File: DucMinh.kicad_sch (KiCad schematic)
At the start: 62 parts, among them J1 Power, J10 HC05, J11 PWR_Selection, J12 BOOT0, J2 M1, J3 USB_B_Micro, J4 M2, J5 M3, J6 AS5600, J7 STLink, J8 Stepper_Motor, SW1 SW_Push, U10 BTS7960B, U2 AMS1117-3.3, U3 LM2596SX-5.0/NOPB, U4 TMC2209_SILENTSTEPSTICK, U5 BTS7960B, U6 STM32F103RCT6, U8 BTS7960B, Y1 8 MHz

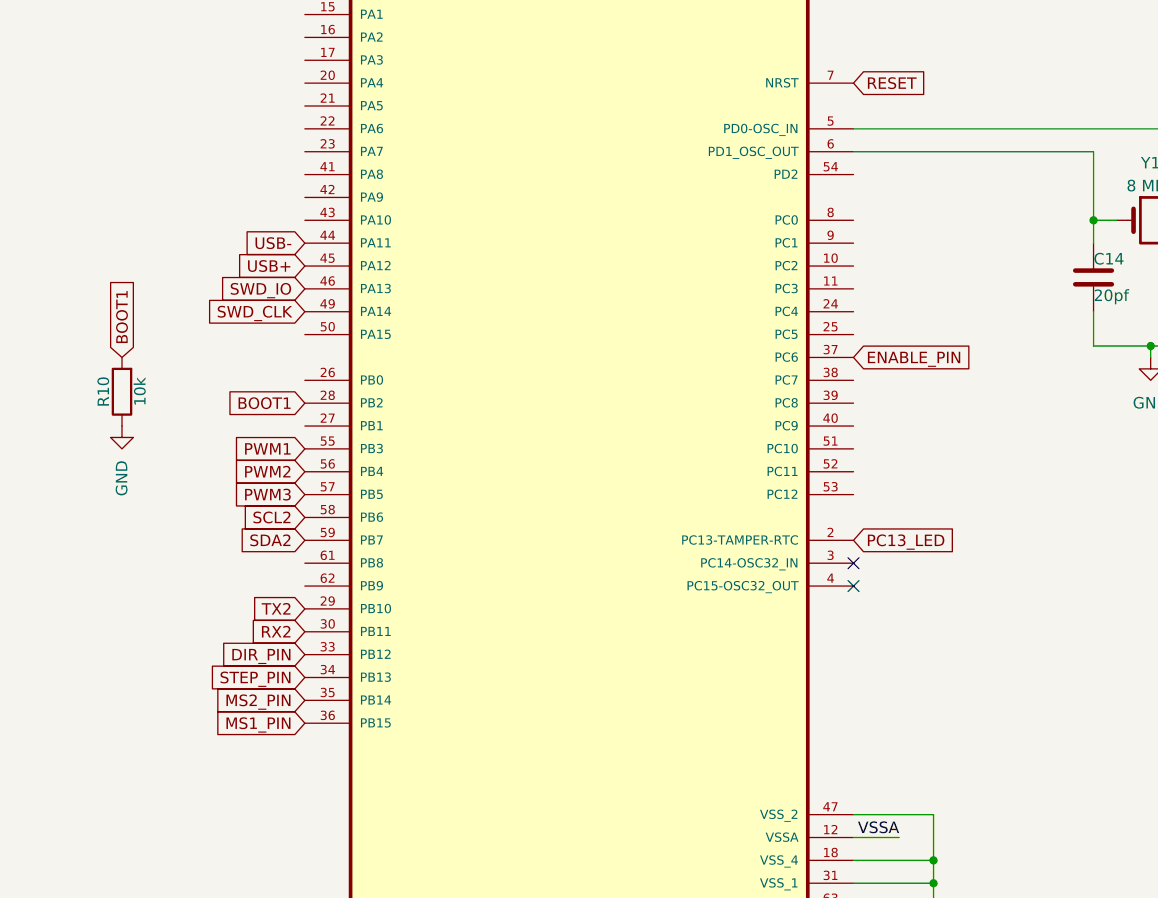
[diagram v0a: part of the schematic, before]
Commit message: final2
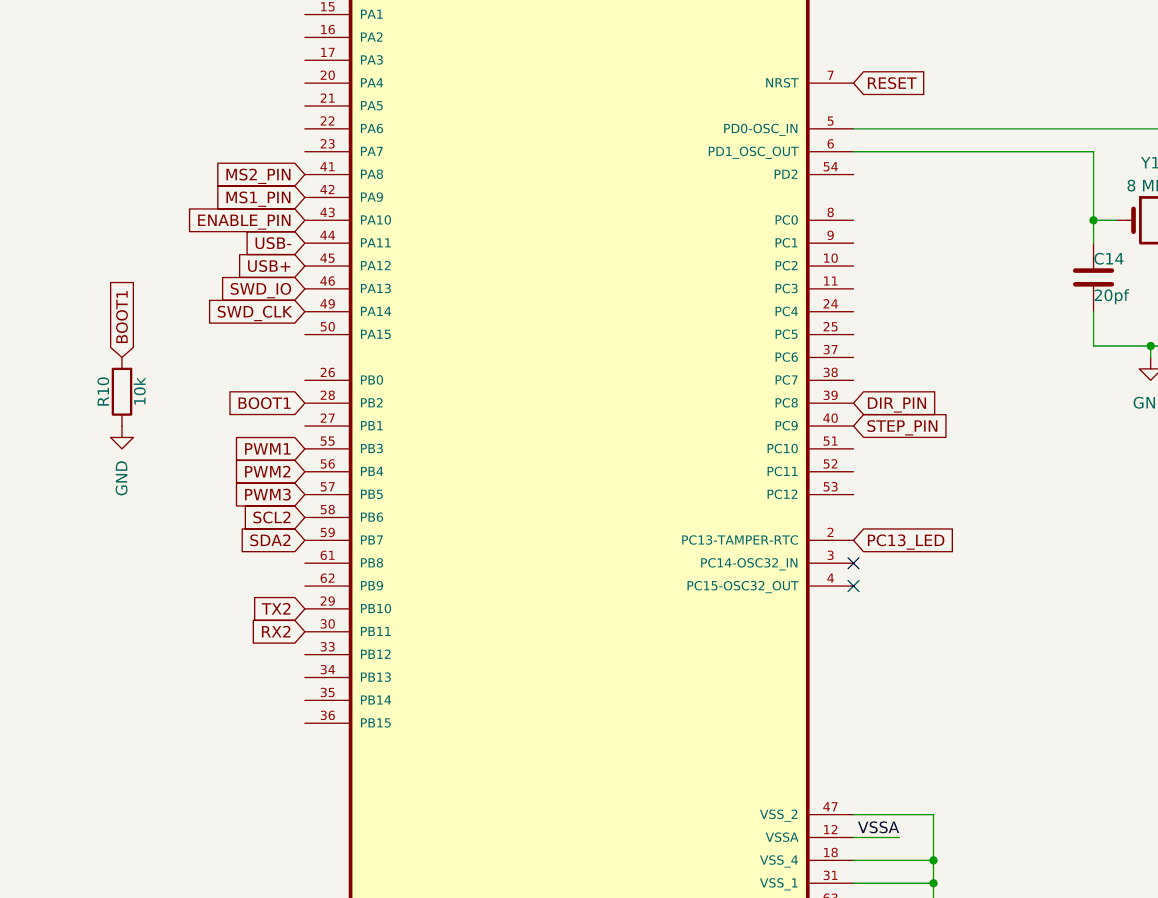
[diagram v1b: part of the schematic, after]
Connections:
- net DIR_PIN: now also U6.39 (PC8); no longer U6.33 (PB12)
- net ENABLE_PIN: now also U6.43 (PA10); no longer U6.37 (PC6)
- net MS1_PIN: now also U6.42 (PA9); no longer U6.36 (PB15)
- net MS2_PIN: now also U6.41 (PA8); no longer U6.35 (PB14)
- net STEP_PIN: now also U6.40 (PC9); no longer U6.34 (PB13)
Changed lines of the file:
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@@
 	(global_label "DIR_PIN"
 		(shape input)
-		(at 283.21 198.12 180)
-		(fields_autoplaced yes)
-		(effects
-			(font
-				(size 1.27 1.27)
-			)
-			(justify right)
-		)
-		(property "Intersheetrefs" "${INTERSHEET_REFS}"
-			(at 272.9071 198.12 0)
-			(effects
-				(font
-					(size 1.27 1.27)
-				)
-				(justify right)
+		(at 344.17 170.18 0)
+		(fields_autoplaced yes)
+		(effects
+			(font
+				(size 1.27 1.27)
+			)
+			(justify left)
+		)
+		(property "Intersheetrefs" "${INTERSHEET_REFS}"
+			(at 354.4729 170.18 0)
+			(effects
+				(font
+					(size 1.27 1.27)
+				)
+				(justify left)
 				(hide yes)
 			)
@@
 	(global_label "STEP_PIN"
 		(shape input)
-		(at 283.21 200.66 180)
-		(fields_autoplaced yes)
-		(effects
-			(font
-				(size 1.27 1.27)
-			)
-			(justify right)
-		)
-		(property "Intersheetrefs" "${INTERSHEET_REFS}"
-			(at 271.4558 200.66 0)
-			(effects
-				(font
-					(size 1.27 1.27)
-				)
-				(justify right)
+		(at 344.17 172.72 0)
+		(fields_autoplaced yes)
+		(effects
+			(font
+				(size 1.27 1.27)
+			)
+			(justify left)
+		)
+		(property "Intersheetrefs" "${INTERSHEET_REFS}"
+			(at 355.9242 172.72 0)
+			(effects
+				(font
+					(size 1.27 1.27)
+				)
+				(justify left)
 				(hide yes)
 			)
@@
 	(global_label "ENABLE_PIN"
 		(shape input)
-		(at 344.17 165.1 0)
-		(fields_autoplaced yes)
-		(effects
-			(font
-				(size 1.27 1.27)
-			)
-			(justify left)
-		)
-		(property "Intersheetrefs" "${INTERSHEET_REFS}"
-			(at 358.3433 165.1 0)
-			(effects
-				(font
-					(size 1.27 1.27)
-				)
-				(justify left)
+		(at 283.21 149.86 180)
+		(fields_autoplaced yes)
+		(effects
+			(font
+				(size 1.27 1.27)
+			)
+			(justify right)
+		)
+		(property "Intersheetrefs" "${INTERSHEET_REFS}"
+			(at 269.0367 149.86 0)
+			(effects
+				(font
+					(size 1.27 1.27)
+				)
+				(justify right)
 				(hide yes)
 			)
@@
 	(global_label "MS2_PIN"
 		(shape input)
-		(at 283.21 203.2 180)
-		(fields_autoplaced yes)
-		(effects
-			(font
-				(size 1.27 1.27)
-			)
-			(justify right)
-		)
-		(property "Intersheetrefs" "${INTERSHEET_REFS}"
-			(at 272.1815 203.2 0)
+		(at 283.21 144.78 180)
+		(fields_autoplaced yes)
+		(effects
+			(font
+				(size 1.27 1.27)
+			)
+			(justify right)
+		)
+		(property "Intersheetrefs" "${INTERSHEET_REFS}"
+			(at 272.1815 144.78 0)
 			(effects
 				(font
@@
 	(global_label "MS1_PIN"
 		(shape input)
-		(at 283.21 205.74 180)
-		(fields_autoplaced yes)
-		(effects
-			(font
-				(size 1.27 1.27)
-			)
-			(justify right)
-		)
-		(property "Intersheetrefs" "${INTERSHEET_REFS}"
-			(at 272.1815 205.74 0)
-			(effects
-				(font
+		(at 283.21 147.32 180)
+		(fields_autoplaced yes)
+		(effects
+			(font
+				(size 1.27 1.27)
+			)
+			(justify right)
+		)
+		(property "Intersheetrefs" "${INTERSHEET_REFS}"
+			(at 272.1815 147.32 0)
+			(effects
+				(font
